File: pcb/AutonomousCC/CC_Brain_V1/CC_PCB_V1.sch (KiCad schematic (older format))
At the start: 19 parts, among them J1 Screw_Terminal_01x07, J2 Antenna_Conn_02x04_Odd_Even, J3 USB1130-15-A_REVA, J5 Relay_Conn_01x06, J9 Conn_01x02_Male, U1 Pico, U2 LM337_TO3

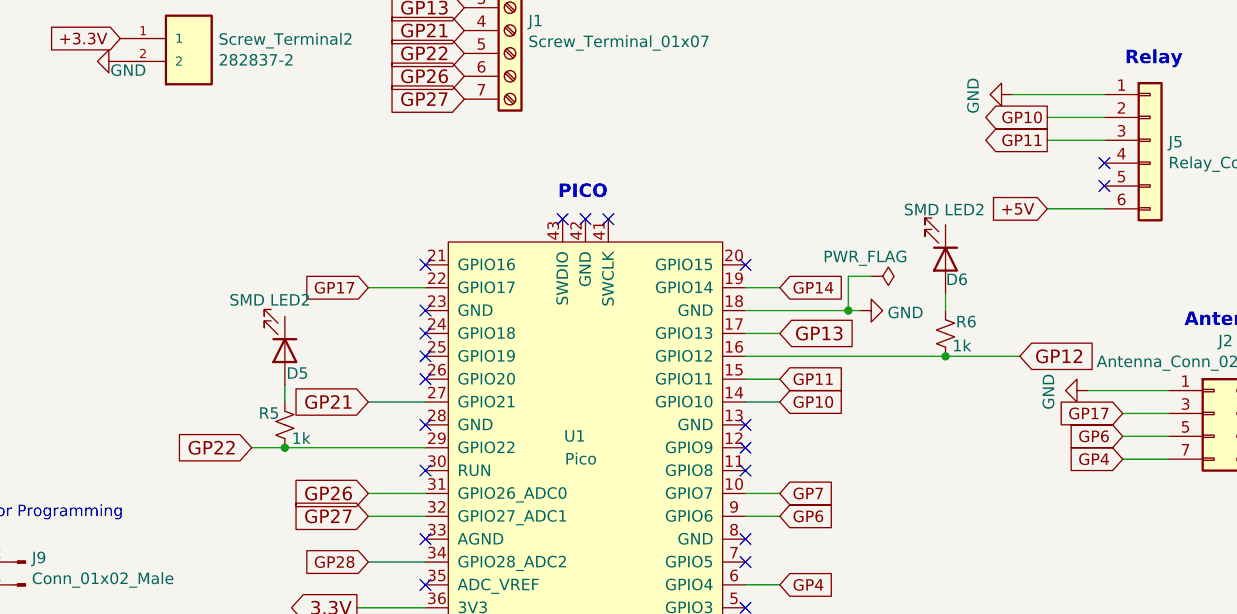
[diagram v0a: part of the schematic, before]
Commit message: CC Controller and Brain VERSION 1.1
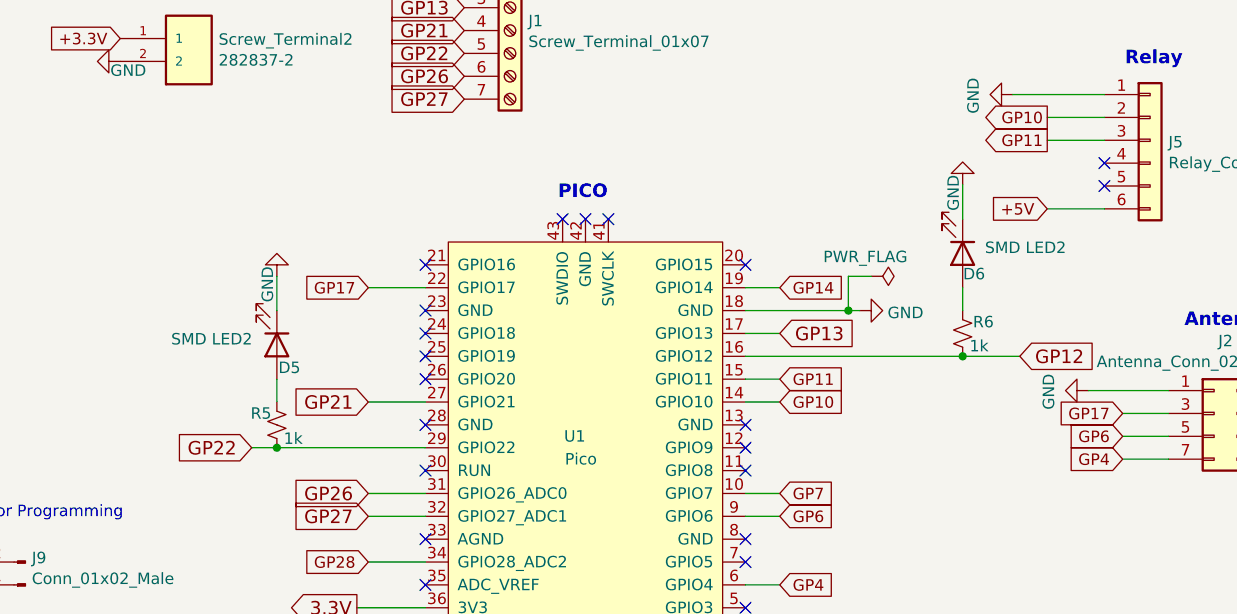
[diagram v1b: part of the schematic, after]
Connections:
- net GND: now also D5.1 (K), D6.1 (K)
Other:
- moved on the sheet: D5, D6, R5, R6
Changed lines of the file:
@@
 L Device:R_Small_US R?
 U 1 1 616756D3
-P 6575 3850
+P 6650 3850
 AR Path="/615DA4AF/616756D3" Ref="R?"  Part="1"
 AR Path="/616756D3" Ref="R6"  Part="1"
-F 0 "R6" H 6620 3900 50  0000 L CNN
-F 1 "1k" H 6605 3795 50  0000 L CNN
-F 2 "Resistor_SMD:R_0603_1608Metric_Pad0.98x0.95mm_HandSolder" H 6575 3850 50  0001 C CNN
-F 3 "~" H 6575 3850 50  0001 C CNN
-	1    6575 3850
+F 0 "R6" H 6695 3900 50  0000 L CNN
+F 1 "1k" H 6680 3795 50  0000 L CNN
+F 2 "Resistor_SMD:R_0603_1608Metric_Pad0.98x0.95mm_HandSolder" H 6650 3850 50  0001 C CNN
+F 3 "~" H 6650 3850 50  0001 C CNN
+	1    6650 3850
 	1    0    0    -1
 $EndComp
@@
 L Device:R_Small_US R?
 U 1 1 61676AAC
-P 3685 4250
+P 3650 4250
 AR Path="/615DA4AF/61676AAC" Ref="R?"  Part="1"
 AR Path="/61676AAC" Ref="R5"  Part="1"
-F 0 "R5" H 3570 4300 50  0000 L CNN
-F 1 "1k" H 3715 4190 50  0000 L CNN
-F 2 "Resistor_SMD:R_0603_1608Metric_Pad0.98x0.95mm_HandSolder" H 3685 4250 50  0001 C CNN
-F 3 "~" H 3685 4250 50  0001 C CNN
-	1    3685 4250
+F 0 "R5" H 3535 4300 50  0000 L CNN
+F 1 "1k" H 3680 4190 50  0000 L CNN
+F 2 "Resistor_SMD:R_0603_1608Metric_Pad0.98x0.95mm_HandSolder" H 3650 4250 50  0001 C CNN
+F 3 "~" H 3650 4250 50  0001 C CNN
+	1    3650 4250
 	1    0    0    -1
 $EndComp
@@
 L Device:LED D?
 U 1 1 616797FD
-P 6575 3525
+P 6650 3500
 AR Path="/615DA4AF/616797FD" Ref="D?"  Part="1"
 AR Path="/616797FD" Ref="D6"  Part="1"
-F 0 "D6" V 6665 3575 50  0000 C CNN
-F 1 "SMD LED2" V 6360 3520 50  0000 C CNN
-F 2 "LED_SMD:LED_1206_3216Metric_Pad1.42x1.75mm_HandSolder" H 6575 3525 50  0001 C CNN
-F 3 "~" H 6575 3525 50  0001 C CNN
-	1    6575 3525
+F 0 "D6" V 6740 3550 50  0000 C CNN
+F 1 "SMD LED2" V 6625 3775 50  0000 C CNN
+F 2 "LED_SMD:LED_1206_3216Metric_Pad1.42x1.75mm_HandSolder" H 6650 3500 50  0001 C CNN
+F 3 "~" H 6650 3500 50  0001 C CNN
+	1    6650 3500
 	0    1    1    0
 $EndComp
@@
 L Device:LED D?
 U 1 1 6167A748
-P 3685 3925
+P 3650 3900
 AR Path="/615DA4AF/6167A748" Ref="D?"  Part="1"
 AR Path="/6167A748" Ref="D5"  Part="1"
-F 0 "D5" V 3785 3980 50  0000 C CNN
-F 1 "SMD LED2" V 3465 3860 50  0000 C CNN
-F 2 "LED_SMD:LED_1206_3216Metric_Pad1.42x1.75mm_HandSolder" H 3685 3925 50  0001 C CNN
-F 3 "~" H 3685 3925 50  0001 C CNN
-	1    3685 3925
+F 0 "D5" V 3750 3955 50  0000 C CNN
+F 1 "SMD LED2" V 3625 3615 50  0000 C CNN
+F 2 "LED_SMD:LED_1206_3216Metric_Pad1.42x1.75mm_HandSolder" H 3650 3900 50  0001 C CNN
+F 3 "~" H 3650 3900 50  0001 C CNN
+	1    3650 3900
 	0    1    1    0
 $EndComp
 Wire Wire Line
-	5700 3950 6575 3950
-Connection ~ 6575 3950
+	3540 4350 3650 4350
+Connection ~ 3650 4350
 Wire Wire Line
-	6575 3950 6900 3950
+	3650 4350 4300 4350
 Wire Wire Line
-	6575 3675 6575 3750
+	3650 4050 3650 4150
+$Comp
+L CC_PCB_V1-rescue:GND-power #PWR?
+U 1 1 616D58BC
+P 3650 3600
+F 0 "#PWR?" H 3650 3350 50  0001 C CNN
+F 1 "GND" V 3690 3635 50  0000 C CNN
+F 2 "" H 3650 3600 50  0001 C CNN
+F 3 "" H 3650 3600 50  0001 C CNN
+	1    3650 3600
+	-1   0    0    1
+$EndComp
 Wire Wire Line
-	3540 4350 3685 4350
-Connection ~ 3685 4350
+	3650 3600 3650 3750
+$Comp
+L CC_PCB_V1-rescue:GND-power #PWR?
+U 1 1 616DC890
+P 6650 3200
+F 0 "#PWR?" H 6650 2950 50  0001 C CNN
+F 1 "GND" V 6690 3235 50  0000 C CNN
+F 2 "" H 6650 3200 50  0001 C CNN
+F 3 "" H 6650 3200 50  0001 C CNN
+	1    6650 3200
+	-1   0    0    1
+$EndComp
+Connection ~ 6650 3950
 Wire Wire Line
-	3685 4350 4300 4350
+	6650 3950 6900 3950
 Wire Wire Line
-	3685 4075 3685 4150
+	5700 3950 6650 3950
+Wire Wire Line
+	6650 3750 6650 3650
+Wire Wire Line
+	6650 3200 6650 3350
 $EndSCHEMATC
